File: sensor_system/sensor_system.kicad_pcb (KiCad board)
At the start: 2 copper layers, 137.1 x 28.5 mm, 57 parts, among them J1 Magnetic connector, J2 Solar_panels, Q1 SBC817, Q2 MJD45H11, SW1 SW_DPDT_x2, U1 TLC555xD, U2 XC6206PxxxMR, U3 MCP73833, U4 BME280, U5 ESP32-DEVKIT-V1, U7 TPS63002

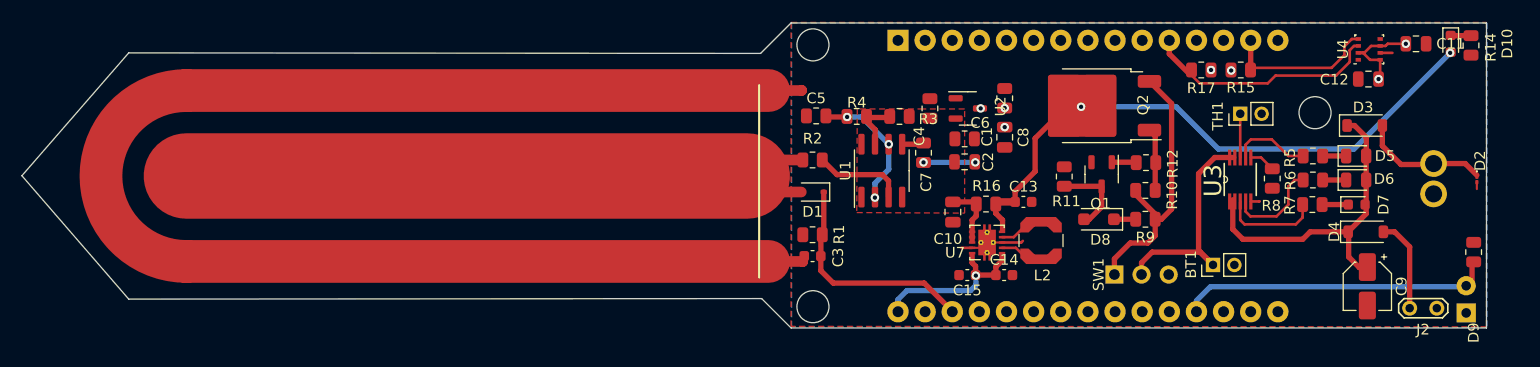
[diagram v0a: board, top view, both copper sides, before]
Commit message: Board fix 2.0
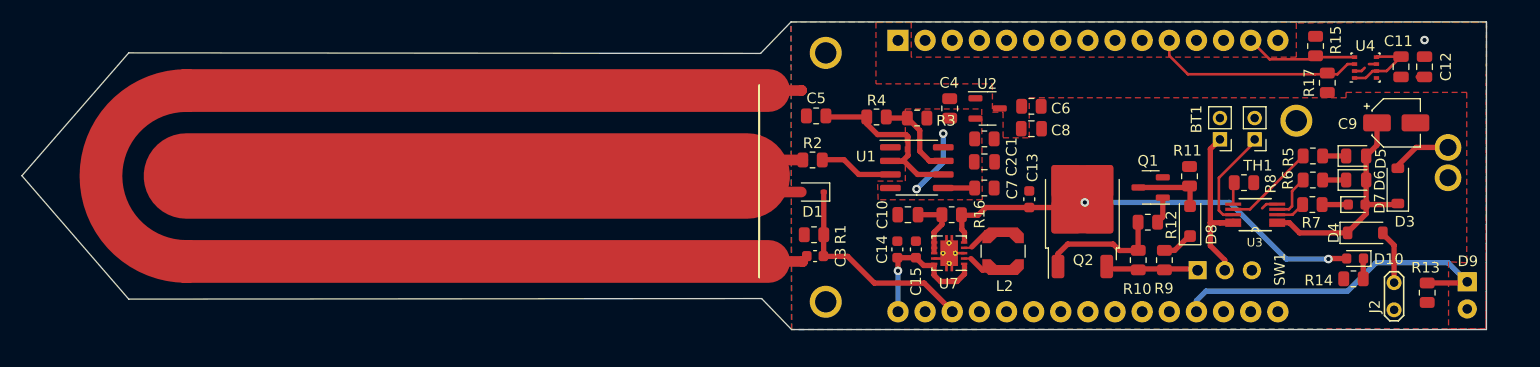
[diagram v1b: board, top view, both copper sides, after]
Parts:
- removed the ? at (143.7, 32.4)
- removed D2: ESD112B102, Diode_SMD:D_01005_0402Metric
- added ?: , , F.Cu at (97.8, 50.1)
- added ?: , , F.Cu at (97.8, 26.8)
- added ?: , , F.Cu at (141.9, 33.1)
- moved R14 24.5 mm to (147.2, 48.0), turned to 0 degrees
- moved D10 22.0 mm to (147.4, 46.0), turned to 180 degrees
- moved C9 15.5 mm to (151.2, 33.4), turned to 0 degrees
- moved R17 11.9 mm to (144.8, 29.6), turned to -90 degrees
- moved BT1 11.8 mm to (134.8, 34.9), turned to 180 degrees
- moved R11 11.7 mm to (131.9, 38.4)
- moved C14 10.3 mm to (104.5, 45.2), turned to 90 degrees
- moved Q2 10.1 mm to (121.9, 41.8), turned to 90 degrees
- moved D8 8.53 mm to (131.9, 42.5), turned to 90 degrees
- moved SW1 7.80 mm to (132.7, 47.1)
- moved R15 7.35 mm to (143.7, 26.2), turned to 90 degrees
- moved C7 6.59 mm to (112.7, 39.5), turned to 0 degrees
- moved R10 6.56 mm to (127.1, 46.2), turned to 90 degrees
- moved D3 6.44 mm to (151.4, 39.2), turned to 90 degrees
- moved R13 5.78 mm to (154.2, 49.2), turned to -90 degrees
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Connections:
- D9 pad 1: 3V3 -> Net-(D9-K)
- D9 pad 2: Net-(D9-A) -> 3V3
- R13 pad 1: Net-(D9-A) -> Net-(D9-K)
- U5 pad 19: Net-(D9-A) -> Net-(D9-K)
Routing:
- net Net-(D9-K): track 0.00 -> 32.6 mm
- net Net-(D9-A): track 30.0 -> 0.00 mm
- net Net-(Q2-E): track 25.9 -> 7.86 mm
- net Net-(D10-A): track 54.4 -> 41.6 mm
- net Net-(D3-K): track 31.0 -> 21.9 mm
- net 3V3: track 9.03 -> 1.84 mm, vias 7 -> 0
- net Net-(U3-STAT1): track 9.22 -> 2.77 mm
- net 3V: track 0.00 -> 6.24 mm, vias 0 -> 2
- net Net-(D3-A): track 12.0 -> 5.83 mm
- net Net-(Q2-B): track 5.87 -> 12.0 mm
- net Net-(U3-THERM): track 4.09 -> 9.65 mm
- net Net-(U1-THR): track 12.8 -> 18.0 mm, vias 3 -> 0
- net Net-(BT1-+): track 22.1 -> 17.1 mm
- net Net-(U3-STAT2): track 8.92 -> 4.39 mm
- net Net-(U1-DIS): track 5.15 -> 9.51 mm
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- added copper zone on F.Cu, net 3V3
- added copper zone on B.Cu, net Earth
- removed copper zone on B.Cu, net 3V3
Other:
- board size 137.1 x 28.5 mm -> 137.1 x 28.8 mm
